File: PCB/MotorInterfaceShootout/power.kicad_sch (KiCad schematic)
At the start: 10 parts, among them U2 OPA4197, U3 LM7810, U4 LM79L05, U5 74LS14, U9 74LS08

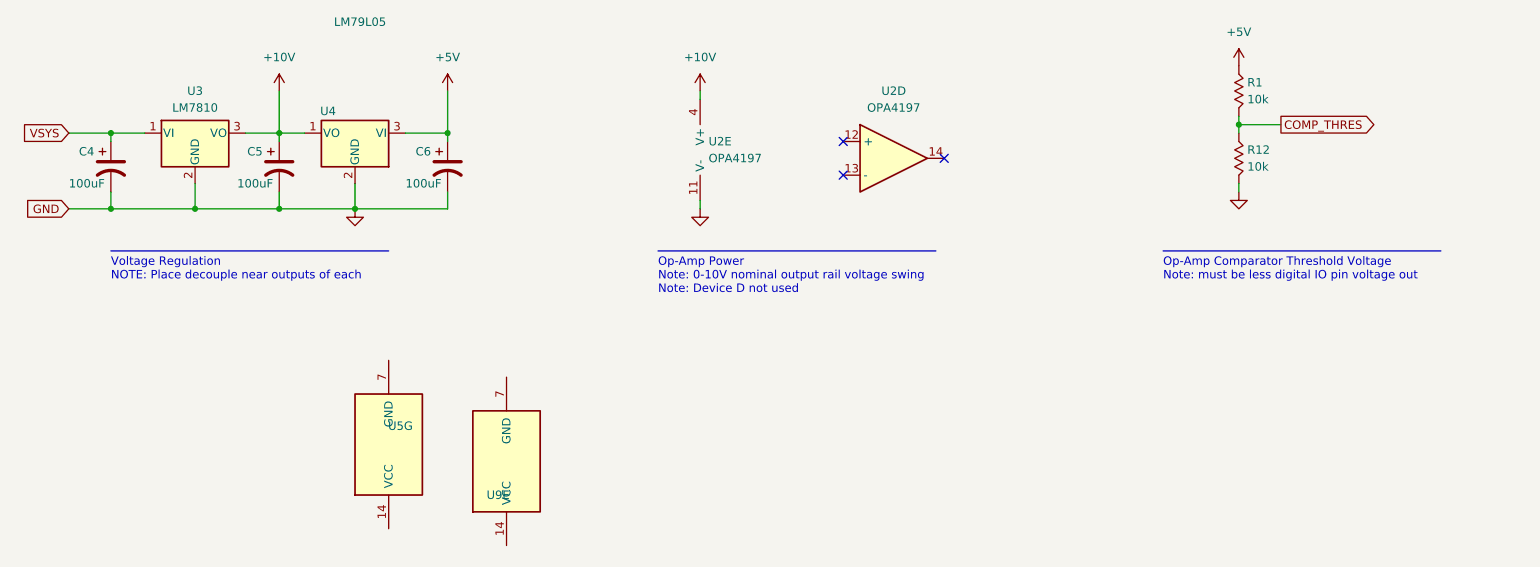
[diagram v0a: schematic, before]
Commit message: working on part source
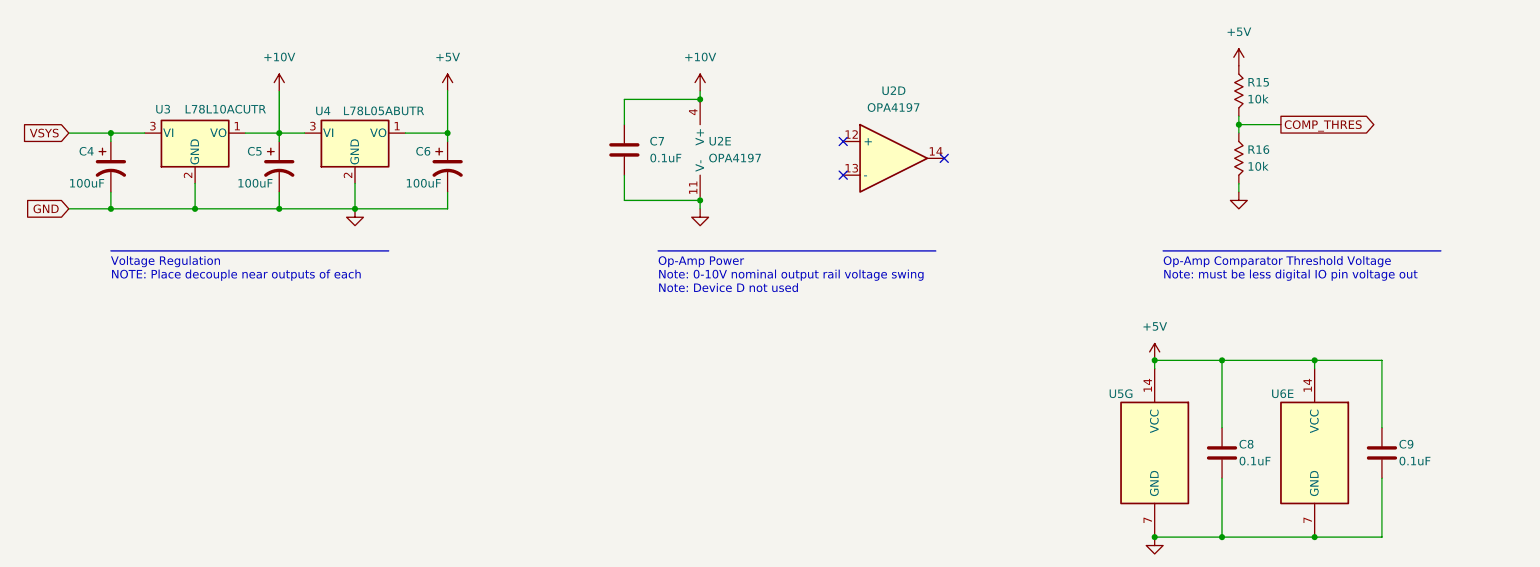
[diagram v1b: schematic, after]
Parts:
- removed U3: LM7810, Package_TO_SOT_THT:TO-220-3_Vertical, symbol Regulator_Linear:LM7810_TO220
- added C7, C8, C9: 0.1uF, symbol device:C
- added U3: L78L10ACUTR, symbol Regulator_Linear:LM78L05_TO92
- C4, C5, C6: footprint TJR:C_Radial_D5.00mm_H12.5mm_P2.00mm -> (none); digikey https://www.digikey.com/en/products/detail/rubycon/16ZLH100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 -> https://www.digikey.com/en/products/detail/nichicon/UWT1V10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
- R15: renamed from R1; footprint TJR:R_Axial_DIN0207_L6.3mm_D2.5mm_P7.62mm_Horizontal -> (none); digikey https://www.digikey.com/en/products/detail/stackpole-electronics-inc/CFM12JT47R0/1741962 -> https://www.digikey.com/en/products/detail/stackpole-electronics-inc/RMCF0805FT10K0/1760676
- R16: renamed from R12; footprint TJR:R_Axial_DIN0207_L6.3mm_D2.5mm_P7.62mm_Horizontal -> (none); digikey https://www.digikey.com/en/products/detail/stackpole-electronics-inc/CFM12JT47R0/1741962 -> https://www.digikey.com/en/products/detail/stackpole-electronics-inc/RMCF0805FT10K0/1760676
- U4: value LM79L05 -> L78L05ABUTR; footprint Package_TO_SOT_THT:TO-92_Inline -> (none); digikey https://www.digikey.com/en/products/detail/texas-instrument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 -> https://www.digikey.com/en/products/detail/stmicroelectroni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
- U5: digikey (none) -> https://www.digikey.com/en/products/detail/texas-instrument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
- U6: renamed from U9; digikey (none) -> https://www.digikey.com/en/products/detail/texas-instrument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
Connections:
- net +10V: now also U4.3 (VI), C7.1, U3.1 (VO); no longer U4.1 (VO)
- net +5V: now also U4.1 (VO), U5.14 (VCC), U6.14 (VCC), C8.1, C9.1; no longer U4.3 (VI)
- net GND: now also U5.7 (GND), U6.7 (GND), C7.2, C8.2, C9.2, U3.2 (GND)
- net VSYS: now also U3.3 (VI)
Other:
- moved on the sheet: U5G, U6E
